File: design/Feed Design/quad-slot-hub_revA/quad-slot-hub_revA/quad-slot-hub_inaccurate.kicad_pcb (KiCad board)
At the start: 2 copper layers, 52 x 52 mm, 5 parts, among them J1 SMA_0732510250

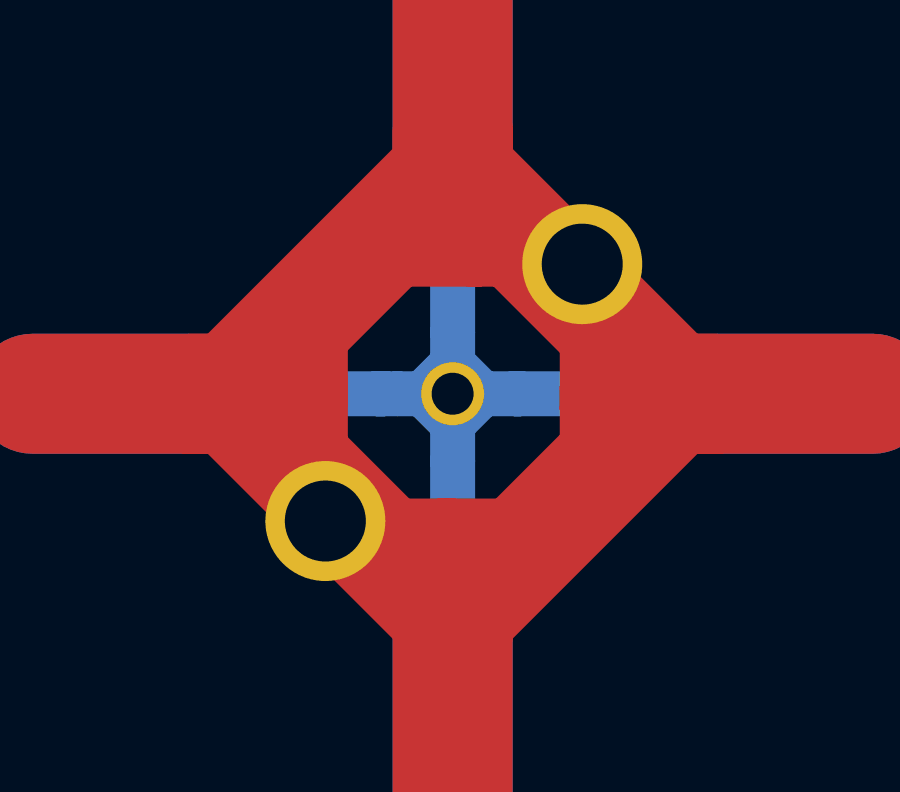
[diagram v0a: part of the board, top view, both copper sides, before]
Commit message: Updated model
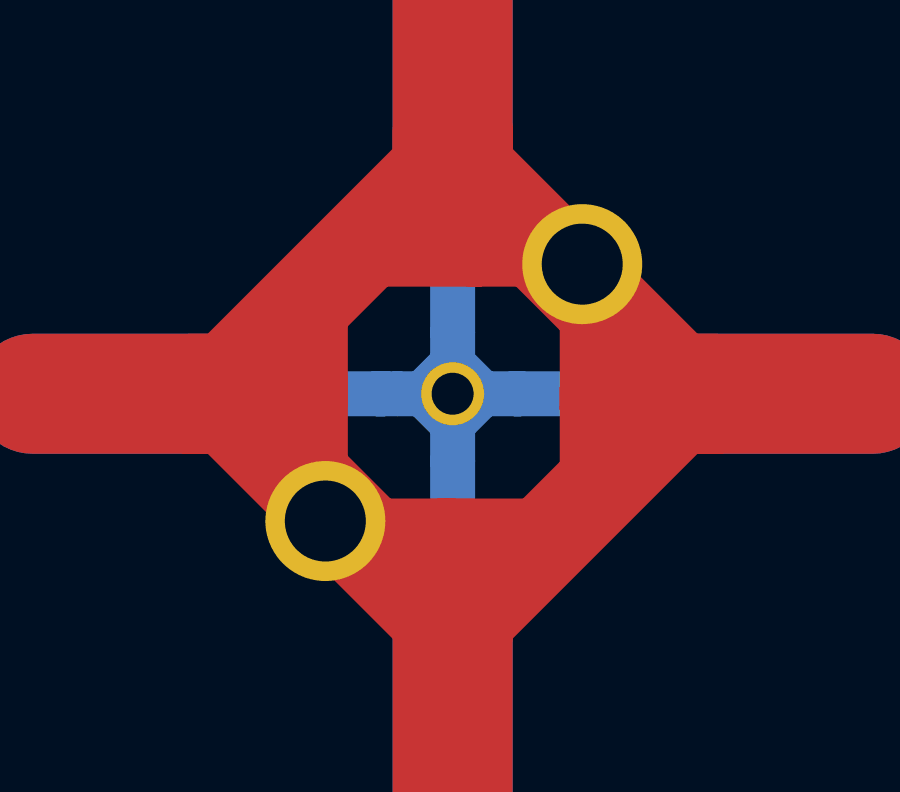
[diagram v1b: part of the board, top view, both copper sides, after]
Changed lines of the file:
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@@
   (segment (start -0.844095 5.03999) (end -1.51001 5.705905) (width 1) (layer F.Cu) (net 2))
   (segment (start 0.12299 5.03999) (end -0.844095 5.03999) (width 1) (layer F.Cu) (net 2))
-  (segment (start 0 6) (end -6 0) (width 1.5) (layer F.Cu) (net 2))
-  (segment (start -6 0) (end 0 -6) (width 1.5) (layer F.Cu) (net 2))
-  (segment (start 0 -6) (end 6 0) (width 1.5) (layer F.Cu) (net 2))
+  (segment (start -0.45 6.175) (end -6.45 0.175) (width 1.5) (layer F.Cu) (net 2))
+  (segment (start -6.55 -0.25) (end -0.55 -6.25) (width 1.5) (layer F.Cu) (net 2))
+  (segment (start 0.375 -6.375) (end 6.375 -0.375) (width 1.5) (layer F.Cu) (net 2))
   (segment (start -0.75 8) (end -8.75 0) (width 2) (layer F.Cu) (net 2))
   (segment (start 0 8) (end -0.75 8) (width 2) (layer F.Cu) (net 2))
@@
   (segment (start -5.63501 -2.88501) (end -5.63501 -1.792669) (width 1.5) (layer F.Cu) (net 2))
   (segment (start 4.257359 4.242641) (end 3 5.5) (width 1.5) (layer F.Cu) (net 2))
-  (segment (start 6 0) (end 0 6) (width 1.5) (layer F.Cu) (net 2))
+  (segment (start 6.375 0.525) (end 0.375 6.525) (width 1.5) (layer F.Cu) (net 2))
 )
